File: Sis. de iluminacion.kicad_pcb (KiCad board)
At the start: 2 copper layers, 88.9 x 98.1 mm, 48 parts, among them J1 Screw_Terminal_01x02, J10 Screw_Terminal_01x02, J11 Screw_Terminal_01x02, J12 Screw_Terminal_01x02, J3 Screw_Terminal_01x02, J4 Conn_01x04, J5 Screw_Terminal_01x02, J7 Screw_Terminal_01x02, J8 Screw_Terminal_01x02, J9 Screw_Terminal_01x02, K10 Relay_DPDT, K11 Relay_DPDT, K8 Relay_DPDT, K9 Relay_DPDT, Q4 BC547, Q5 BC547, Q6 BC547, Q7 BC547, U1 ESP32_DEVKITC, U10 PC817, U11 PC817, U12 PC817, U13 PC817, U3 L7805

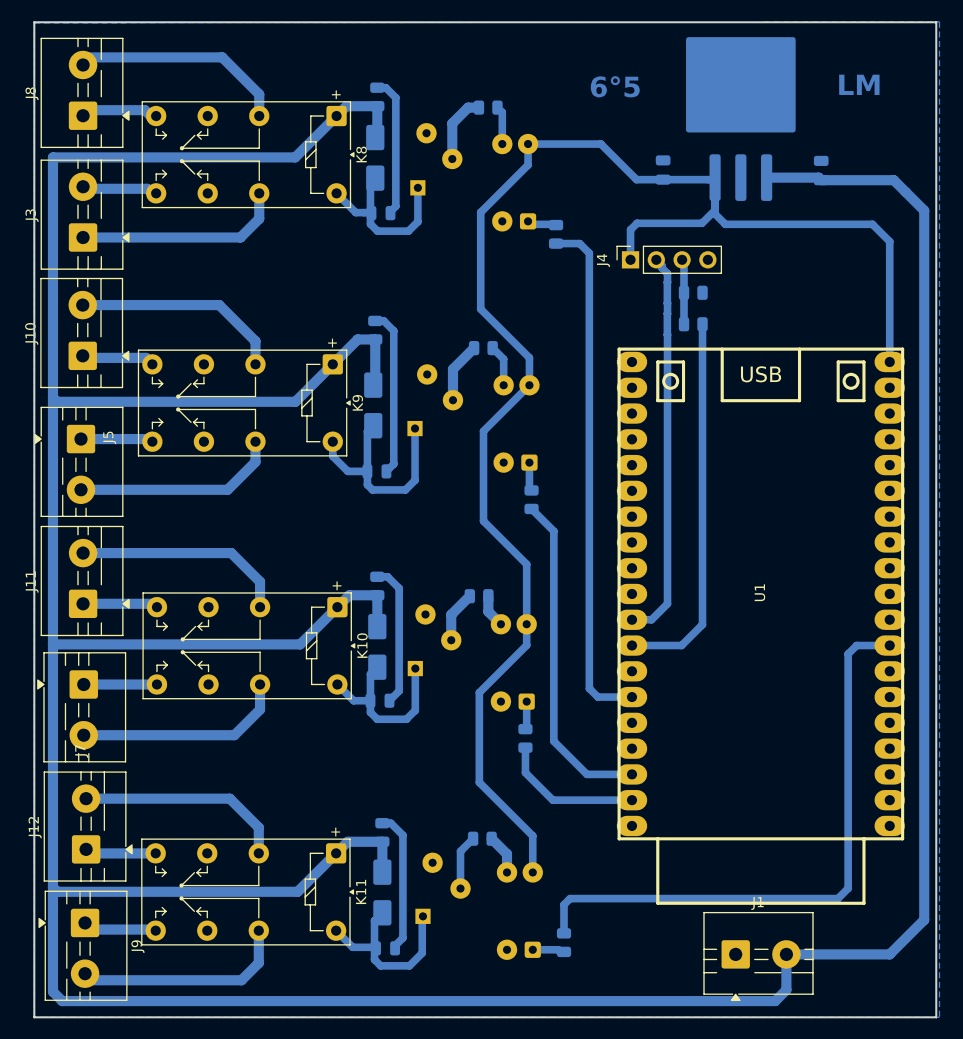
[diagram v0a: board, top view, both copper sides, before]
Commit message: Add files via upload
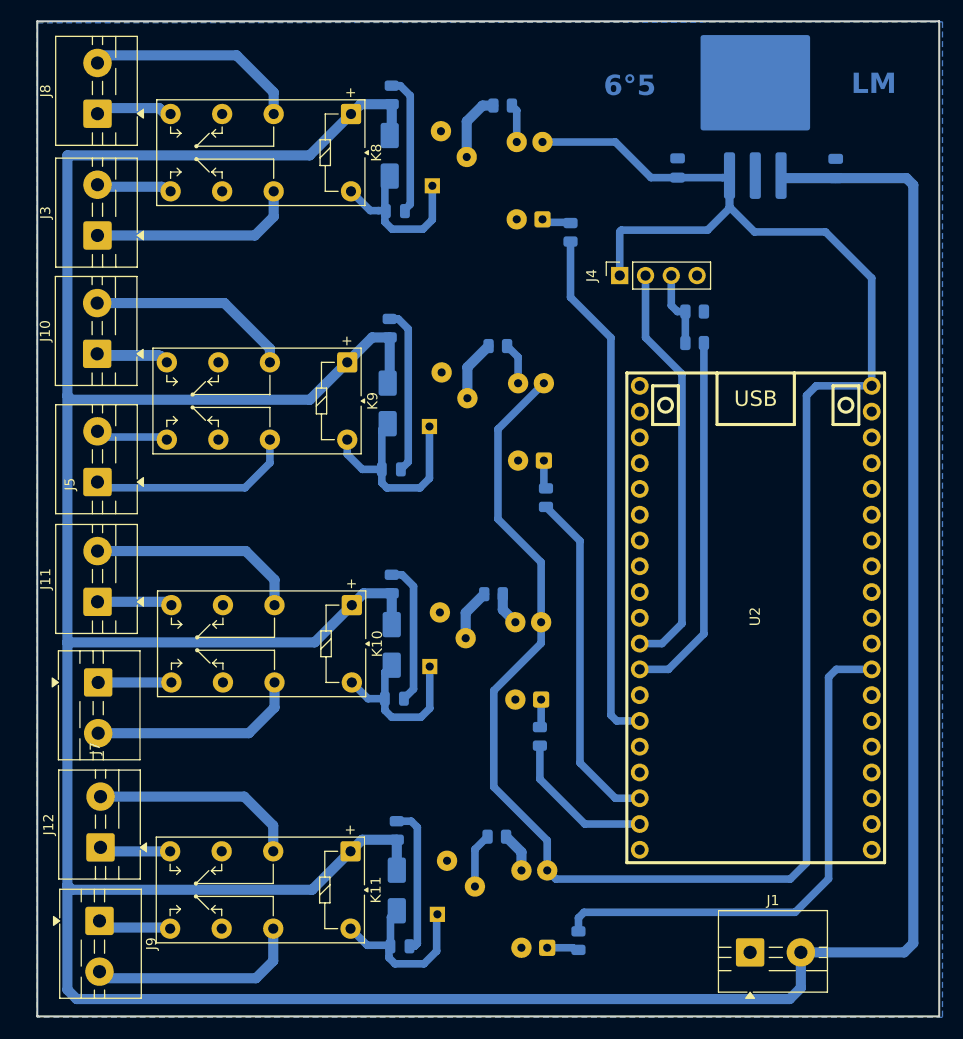
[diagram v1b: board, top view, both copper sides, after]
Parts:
- removed U1: ESP32_DEVKITC, EESTN5:ESP32_DEVKITC
- added U2: ESP32_DEVKITC, EESTN5:ESP32S, F.Cu at (250.9, 100.3)
- moved J5 4.54 mm to (186.0, 87.0), turned to 90 degrees
- moved J4 1.88 mm to (237.5, 66.6)
- moved R17 1.85 mm to (244.9, 70.2)
- moved R16 1.85 mm to (244.9, 73.2)
- moved D21 1.44 mm to (215.8, 132.7)
- moved R36 1.44 mm to (233.4, 132.1)
- moved D17 1.44 mm to (215.0, 85.7)
- moved D18 1.44 mm to (214.6, 79.2)
- moved D20 1.44 mm to (215.0, 103.0)
- moved D22 1.44 mm to (215.5, 127.2)
- moved J10 1.44 mm to (186.0, 74.3)
- moved J11 1.44 mm to (186.0, 98.8)
- moved J3 1.44 mm to (186.0, 62.6)
- moved J7 1.44 mm to (186.1, 106.7)
- moved J8 1.44 mm to (186.0, 50.6)
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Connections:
- J5 pad 1: NO1 -> V1
- J5 pad 2: V1 -> NO1
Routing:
- net +5V: track 152.5 -> 205.1 mm
- net NO9: track 7.67 -> 14.9 mm
- net GIOP33: track 59.0 -> 52.0 mm
- net GIOP18: track 38.5 -> 40.8 mm
- net +12V: track 411.7 -> 409.6 mm
- net Net-(J4-Pin_3): track 6.43 -> 7.69 mm
- net GIOP22: track 32.9 -> 33.9 mm
- net GIOP19: track 37.4 -> 36.4 mm
- net GIOP23: track 14.1 -> 15.0 mm
- net Net-(D21-A): track 14.0 -> 14.6 mm
- net COM9: track 20.8 -> 20.2 mm
